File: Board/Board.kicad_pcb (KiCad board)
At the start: 2 copper layers, 13 parts, among them J1 Conn_01x12_Male, Q1 Q_PNP_BCEC, U1 ADAU1701

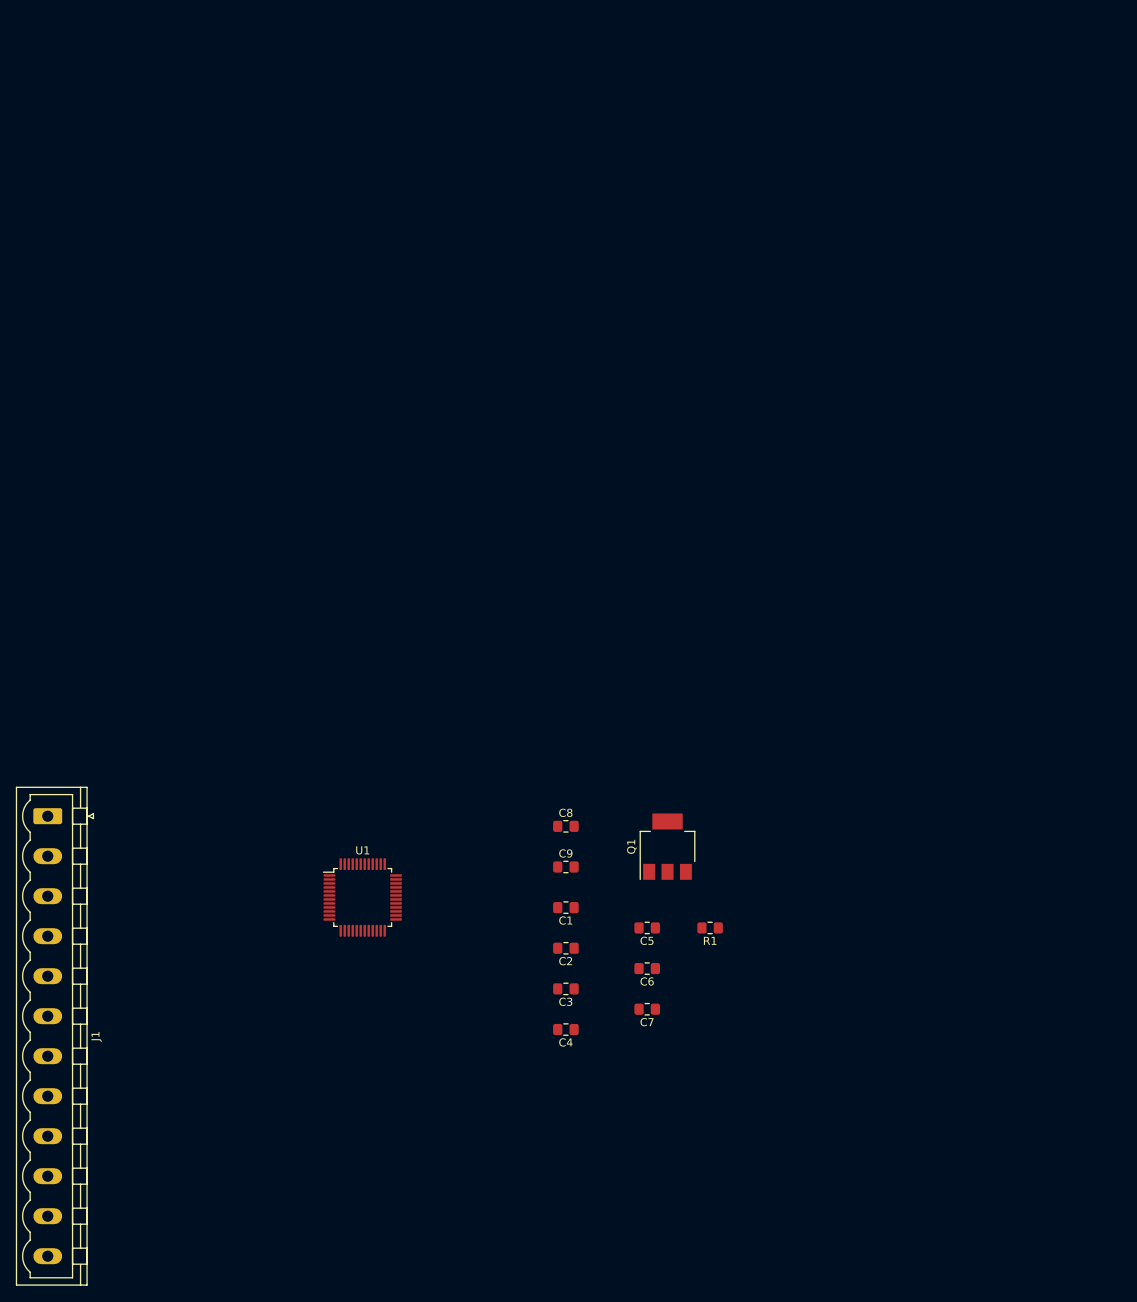
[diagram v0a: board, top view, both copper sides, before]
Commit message: did some more stuff
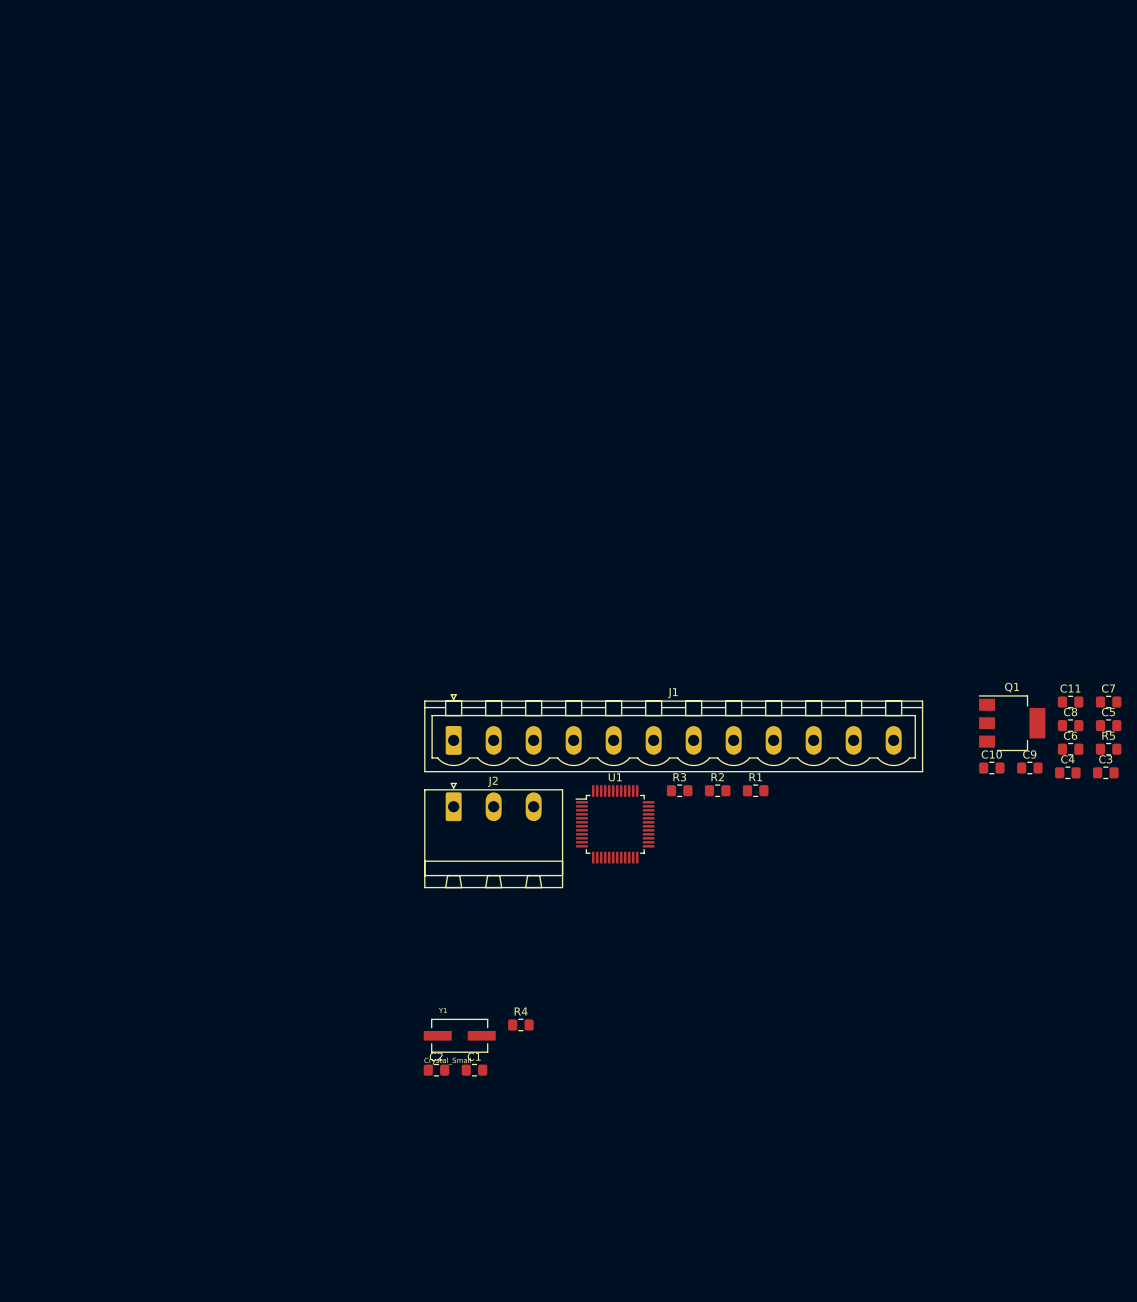
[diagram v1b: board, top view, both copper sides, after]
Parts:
- added C10: 100nF, Capacitor_SMD:C_0805_2012Metric_Pad1.15x1.40mm_HandSolder, F.Cu at (137.1, 32.1)
- added C11: 100nF, Capacitor_SMD:C_0805_2012Metric_Pad1.15x1.40mm_HandSolder, F.Cu at (146.9, 23.8)
- added J2: Audio In, Connector_Phoenix_MSTB:PhoenixContact_MSTBA_2,5_3-G_1x03_P5.00mm_Horizontal, F.Cu at (69.8, 36.9)
- added R2: 18k0, Resistor_SMD:R_0805_2012Metric_Pad1.15x1.40mm_HandSolder, F.Cu at (102.8, 34.9)
- added R3: 18k0, Resistor_SMD:R_0805_2012Metric_Pad1.15x1.40mm_HandSolder, F.Cu at (98.0, 34.9)
- added R4: 100, Resistor_SMD:R_0805_2012Metric_Pad1.15x1.40mm_HandSolder, F.Cu at (78.2, 64.2)
- added R5: 1k00, Resistor_SMD:R_0805_2012Metric_Pad1.15x1.40mm_HandSolder, F.Cu at (151.7, 29.7)
- added Y1: Crystal_Small, ECS-122.8-20-3X-EN-TR:XTAL_ECS-122.8-20-3X-EN-TR, F.Cu at (70.5, 65.5)
- C1, C2: value 100nF -> 22pF
- C4, C5, C8: value 10nF -> 100nF
- C6, C7, C9: value 100nF -> 10nF
- R1: value 1k00 -> 18k
- moved C3 72.7 mm to (151.3, 32.7), turned to 0 degrees
- moved C4 70.5 mm to (146.6, 32.7), turned to 0 degrees
- moved C7 69.3 mm to (151.7, 23.8), turned to 0 degrees
- moved C8 64.3 mm to (146.9, 26.8)
- moved C5 63.0 mm to (151.7, 26.8), turned to 0 degrees
- moved C6 59.6 mm to (146.9, 29.7), turned to 0 degrees
- moved C9 59.3 mm to (141.8, 32.1)
- moved J1 51.6 mm to (69.8, 28.6), turned to 0 degrees
- moved Q1 45.8 mm to (139.6, 26.5), turned to 0 degrees
- moved U1 32.9 mm to (90.0, 39.1)
- moved C1 23.3 mm to (72.4, 69.8), turned to 0 degrees
- moved C2 22.2 mm to (67.6, 69.8), turned to 0 degrees
- moved R1 18.1 mm to (107.5, 34.9), turned to 0 degrees
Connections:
- C1 pad 1: VDD -> GND
- C1 pad 2: GND -> Net-(C1-Pad2)
- C2 pad 1: VDD -> GND
- C2 pad 2: GND -> /oscillator/MCLKI
- C5 pad 1: GND -> VDD
- C5 pad 2: Net-(C5-Pad2) -> GND
- C6 pad 1: GND -> VDD
- C6 pad 2: Net-(C5-Pad2) -> GND
- C7 pad 2: Net-(C5-Pad2) -> VDD
- C9 pad 2: VDD -> /power/DVDD
- Q1 pad 1: Net-(Q1-Pad1) -> /power/VDRIVE
- Q1 pad 2: Net-(C5-Pad2) -> /power/DVDD
- Q1 pad 4: Net-(C5-Pad2) -> /power/DVDD
- R1 pad 1: VDD -> Net-(R1-Pad1)
- R1 pad 2: Net-(Q1-Pad1) -> GND
- U1 pad 1: Net-(U1-Pad1) -> GND
- U1 pad 12: Net-(U1-Pad12) -> GND
- U1 pad 13: Net-(C5-Pad2) -> /power/DVDD
- U1 pad 17: Net-(Q1-Pad1) -> /power/VDRIVE
- U1 pad 24: Net-(C5-Pad2) -> /power/DVDD
- U1 pad 25: Net-(U1-Pad12) -> GND
- U1 pad 3: Net-(U1-Pad3) -> Net-(R1-Pad1)
- U1 pad 30: Net-(U1-Pad30) -> GND
- U1 pad 31: Net-(U1-Pad31) -> /oscillator/OSCO
- U1 pad 32: Net-(U1-Pad32) -> /oscillator/MCLKI
- U1 pad 33: Net-(U1-Pad33) -> GND
- U1 pad 37: Net-(U1-Pad1) -> GND
- U1 pad 42: Net-(U1-Pad1) -> GND

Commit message: more improvements
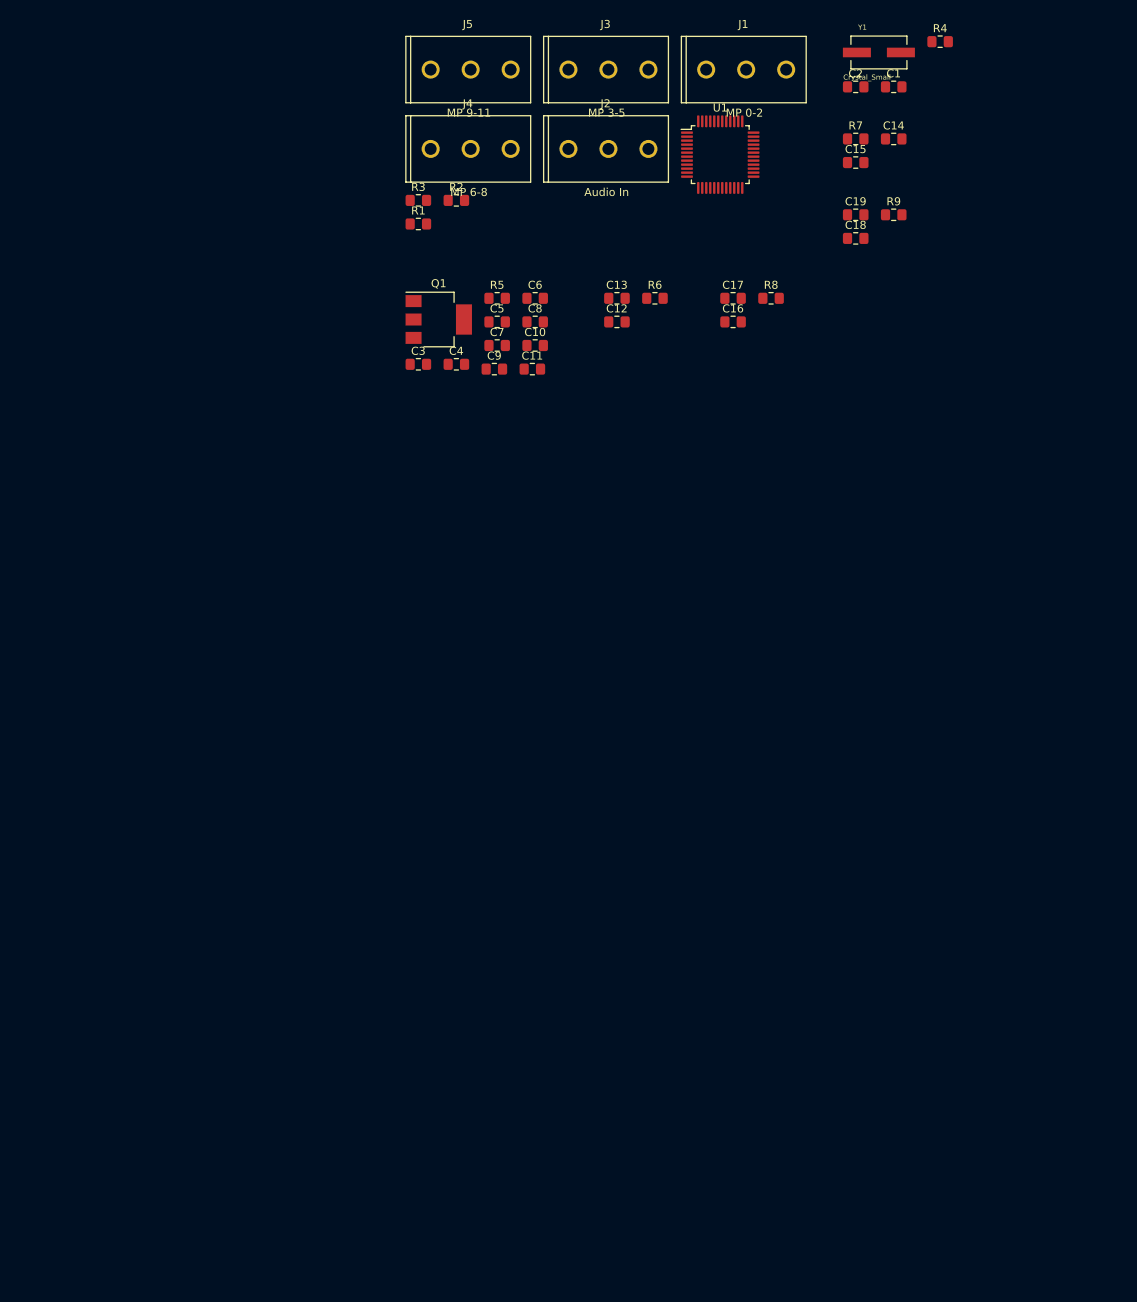
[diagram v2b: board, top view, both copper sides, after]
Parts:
- added C12: 47uF, Capacitor_SMD:C_0805_2012Metric_Pad1.15x1.40mm_HandSolder, F.Cu at (90.2, -23.7)
- added C13: 5n6F, Capacitor_SMD:C_0805_2012Metric_Pad1.15x1.40mm_HandSolder, F.Cu at (90.2, -26.6)
- added C14: 47uF, Capacitor_SMD:C_0805_2012Metric_Pad1.15x1.40mm_HandSolder, F.Cu at (124.8, -46.6)
- added C15: 5n6F, Capacitor_SMD:C_0805_2012Metric_Pad1.15x1.40mm_HandSolder, F.Cu at (120.0, -43.6)
- added C16: 47uF, Capacitor_SMD:C_0805_2012Metric_Pad1.15x1.40mm_HandSolder, F.Cu at (104.7, -23.7)
- added C17: 5n6F, Capacitor_SMD:C_0805_2012Metric_Pad1.15x1.40mm_HandSolder, F.Cu at (104.7, -26.6)
- added C18: 47uF, Capacitor_SMD:C_0805_2012Metric_Pad1.15x1.40mm_HandSolder, F.Cu at (120.0, -34.1)
- added C19: 5n6F, Capacitor_SMD:C_0805_2012Metric_Pad1.15x1.40mm_HandSolder, F.Cu at (120.0, -37.1)
- added J3: MP 3-5, 691213710003:691213710003, F.Cu at (89.1, -55.2)
- added J4: MP 6-8, 691213710003:691213710003, F.Cu at (71.9, -45.3)
- added J5: MP 9-11, 691213710003:691213710003, F.Cu at (71.9, -55.2)
- added R6: 560r, Resistor_SMD:R_0805_2012Metric_Pad1.15x1.40mm_HandSolder, F.Cu at (94.9, -26.6)
- added R7: 560r, Resistor_SMD:R_0805_2012Metric_Pad1.15x1.40mm_HandSolder, F.Cu at (120.0, -46.6)
- added R8: 560r, Resistor_SMD:R_0805_2012Metric_Pad1.15x1.40mm_HandSolder, F.Cu at (109.5, -26.6)
- added R9: 560r, Resistor_SMD:R_0805_2012Metric_Pad1.15x1.40mm_HandSolder, F.Cu at (124.8, -37.1)
- J1: value Conn_01x12_Male -> MP 0-2; footprint Connector_Phoenix_MSTB:PhoenixContact_MSTBVA_2,5_12-G_1x12_P5.00mm_Vertical -> 691213710003:691213710003
- J2: footprint Connector_Phoenix_MSTB:PhoenixContact_MSTBA_2,5_3-G_1x03_P5.00mm_Horizontal -> 691213710003:691213710003
- moved C1 133.6 mm to (124.8, -53.1)
- moved C2 133.6 mm to (120.0, -53.1)
- moved R4 133.6 mm to (130.6, -58.7)
- moved Y1 133.6 mm to (122.9, -57.4)
- moved C3 100.0 mm to (65.4, -18.4)
- moved R5 95.0 mm to (75.2, -26.6)
- moved C4 91.9 mm to (70.1, -18.4)
- moved C5 91.6 mm to (75.2, -23.7)
- moved J1 91.5 mm to (106.4, -55.2)
- moved C7 88.5 mm to (75.2, -20.7)
- moved Q1 87.7 mm to (67.9, -24.0)
- moved C6 87.5 mm to (80.0, -26.6)
- moved U1 84.7 mm to (103.1, -44.6)
- moved J2 84.5 mm to (89.1, -45.3)
- moved C8 83.8 mm to (80.0, -23.7)
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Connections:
- J2 pad 3: GND -> Net-(J2-Pad3)
- R2 pad 2: Net-(J2-Pad1) -> Net-(R2-Pad2)
- R3 pad 2: Net-(J2-Pad2) -> Net-(R3-Pad2)
- U1 pad 10: Net-(J1-Pad11) -> Net-(J1-Pad2)
- U1 pad 11: Net-(J1-Pad12) -> Net-(J1-Pad1)
- U1 pad 14: Net-(J1-Pad5) -> Net-(J4-Pad2)
- U1 pad 15: Net-(J1-Pad6) -> Net-(J4-Pad1)
- U1 pad 16: Net-(J1-Pad2) -> Net-(J5-Pad2)
- U1 pad 19: Net-(J1-Pad1) -> Net-(J5-Pad3)
- U1 pad 26: Net-(J1-Pad3) -> Net-(J5-Pad1)
- U1 pad 27: Net-(J1-Pad4) -> Net-(J4-Pad3)
- U1 pad 28: Net-(J1-Pad9) -> Net-(J3-Pad1)
- U1 pad 29: Net-(J1-Pad10) -> Net-(J1-Pad3)
- U1 pad 43: Net-(U1-Pad43) -> /output filter  4/In
- U1 pad 44: Net-(U1-Pad44) -> /output filter 3/In
- U1 pad 45: Net-(U1-Pad45) -> /output filter 2/In
- U1 pad 46: Net-(U1-Pad46) -> /output filter 1/In
- U1 pad 8: Net-(J1-Pad8) -> Net-(J3-Pad2)
- U1 pad 9: Net-(J1-Pad7) -> Net-(J3-Pad3)
